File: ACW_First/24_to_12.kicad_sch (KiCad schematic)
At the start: 19 parts, among them U1 MP1584EN

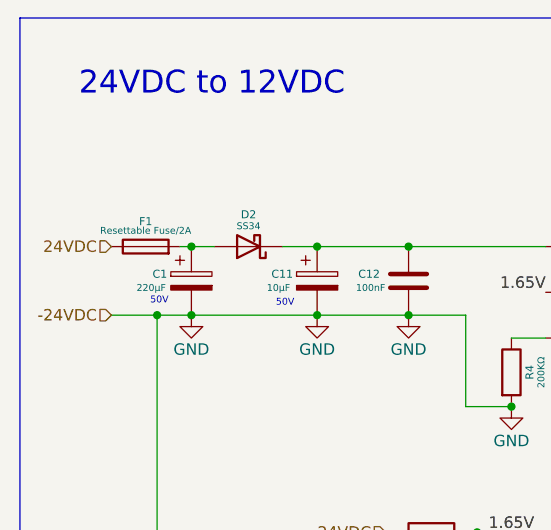
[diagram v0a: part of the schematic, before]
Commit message: okok
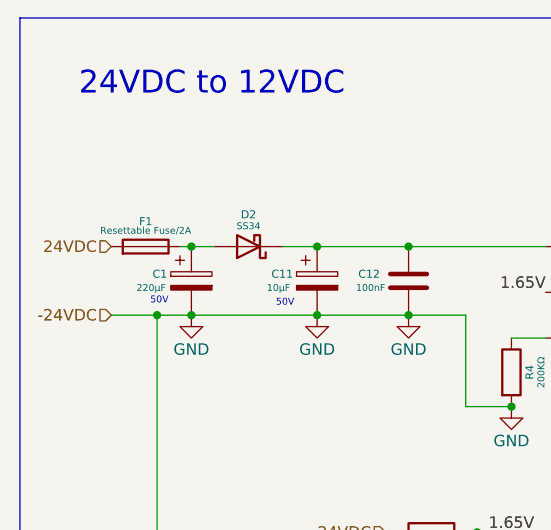
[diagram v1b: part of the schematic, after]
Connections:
- net 24VDC: now also F1.2; no longer F1.1
- net at C1.1, D2.2 (A): now also F1.1; no longer F1.2
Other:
- moved on the sheet: F1
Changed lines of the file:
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@@
 	(symbol
 		(lib_id "Device:Fuse")
-		(at 71.12 68.58 90)
+		(at 71.12 68.58 270)
+		(mirror x)
 		(unit 1)
 		(body_style 1)
